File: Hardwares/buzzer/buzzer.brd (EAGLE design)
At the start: 95.5 x 82.6 mm, 5 parts, among them U1 ARDUINO-UNO-R3-SHIELD

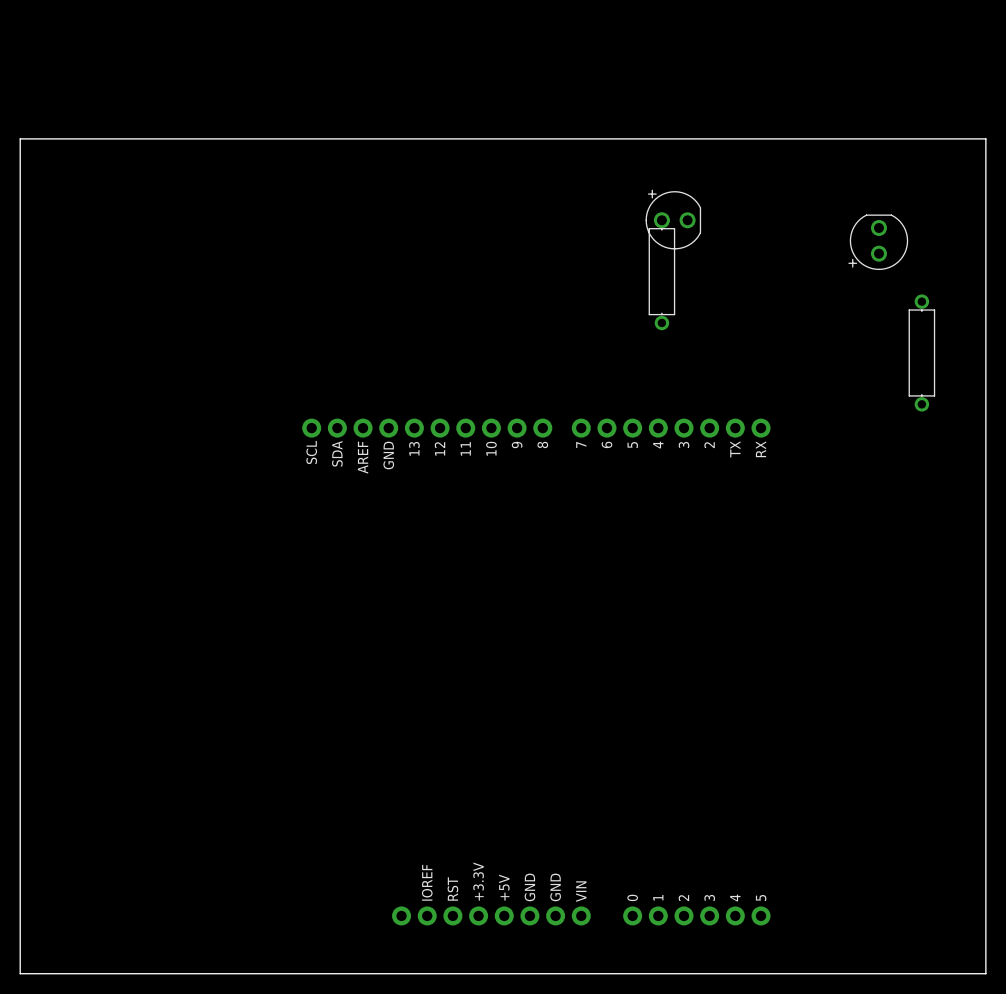
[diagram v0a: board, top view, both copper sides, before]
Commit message: brd csv html pdf png url ino
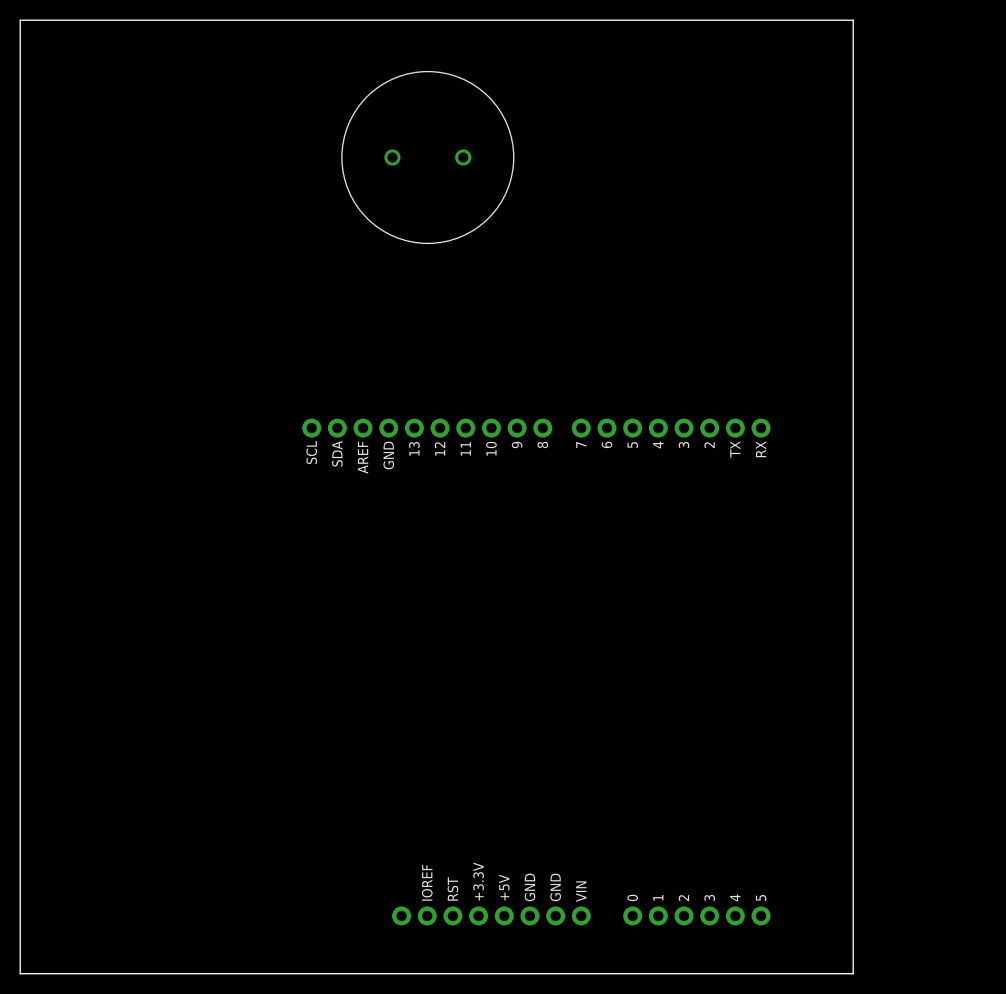
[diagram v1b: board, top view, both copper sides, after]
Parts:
- removed D1: GREEN, Tinkercad:LEDRD254W60D565H860B_G
- removed D2: RED, Tinkercad:LEDRD254W60D565H860B
- removed R1: 200, Tinkercad:RESAD1016W63L850D250B
- removed R2: 1k, Tinkercad:RESAD1016W63L850D250B
- added PIEZO1: PIEZO, Tinkercad:PIEZO
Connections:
- removed net D1_A: D1.1, R2.2
- removed net D2_A: D2.1, R1.1
- removed net U1_RX: R1.2, R2.1, U1.RX
- new net U1_D12: PIEZO1.1, U1.D12
- net U1_GND: now also PIEZO1.2; no longer D1.2, D2.2
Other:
- board size 95.5 x 82.6 mm -> 82.4 x 94.3 mm
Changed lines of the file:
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@@
 <board>
 <plain>
-<wire x1="0" y1="0" x2="95.52872003241336" y2="0" width="0" layer="20"/>
-<wire x1="95.52872003241336" y1="0" x2="95.52872003241336" y2="82.58300179113014" width="0" layer="20"/>
-<wire x1="95.52872003241336" y1="82.58300179113014" x2="0" y2="82.58300179113014" width="0" layer="20"/>
-<wire x1="0" y1="82.58300179113014" x2="0" y2="0" width="0" layer="20"/>
+<wire x1="0" y1="0" x2="82.40360000000003" y2="0" width="0" layer="20"/>
+<wire x1="82.40360000000003" y1="0" x2="82.40360000000003" y2="94.3253326403326" width="0" layer="20"/>
+<wire x1="82.40360000000003" y1="94.3253326403326" x2="0" y2="94.3253326403326" width="0" layer="20"/>
+<wire x1="0" y1="94.3253326403326" x2="0" y2="0" width="0" layer="20"/>
 </plain>
 <attributes/>
@@
 </autorouter>
 <elements>
-<element name="D2" library="Tinkercad" package="LEDRD254W60D565H860B" package3d_urn="urn:adsk.eagle:package:16378508/1" value="RED" x="64.7508" y="74.5334" rot="R360" smashed="yes">
-<attribute name="CATEGORY" value="Opto-Electronic" x="64.7508" y="74.5334" size="1.778" layer="27" display="off"/>
-<attribute name="COLOR" value="" x="64.7508" y="74.5334" size="1.778" layer="27" display="off"/>
-<attribute name="DESCRIPTION" value="" x="64.7508" y="74.5334" size="1.778" layer="27" display="off"/>
-<attribute name="MANUFACTURER" value="" x="64.7508" y="74.5334" size="1.778" layer="27" display="off"/>
-<attribute name="MPN" value="" x="64.7508" y="74.5334" size="1.778" layer="27" display="off"/>
-<attribute name="OPERATING_TEMP" value="" x="64.7508" y="74.5334" size="1.778" layer="27" display="off"/>
-<attribute name="PART_STATUS" value="" x="64.7508" y="74.5334" size="1.778" layer="27" display="off"/>
-<attribute name="ROHS_COMPLIANT" value="" x="64.7508" y="74.5334" size="1.778" layer="27" display="off"/>
-<attribute name="SERIES" value="" x="64.7508" y="74.5334" size="1.778" layer="27" display="off"/>
-<attribute name="SUB-CATEGORY" value="LED" x="64.7508" y="74.5334" size="1.778" layer="27" display="off"/>
-<attribute name="THERMALLOSS" value="" x="64.7508" y="74.5334" size="1.778" layer="27" display="off"/>
-<attribute name="TYPE" value="" x="64.7508" y="74.5334" size="1.778" layer="27" display="off"/>
-<attribute name="VALUE" value="LED_RED" x="64.7508" y="74.5334" size="1.778" layer="27" display="off"/>
-</element>
-<element name="R1" library="Tinkercad" package="RESAD1016W63L850D250B" package3d_urn="urn:adsk.eagle:package:31513020/1" value="200" x="63.4808" y="69.4534" rot="R270" smashed="yes"/>
+<element name="PIEZO1" library="Tinkercad" package="PIEZO" package3d_urn="urn:adsk.eagle:package:32623992/1" value="PIEZO" x="40.323" y="80.7453" rot="R180" smashed="yes"/>
 <element name="U1" library="Tinkercad" package="ARDUINO-UNO-R3-SHIELD" package3d_urn="urn:adsk.eagle:package:32092383/3" value="ARDUINO-UNO-R3-SHIELD" x="47.885" y="29.845" rot="R270" smashed="yes"/>
-<element name="D1" library="Tinkercad" package="LEDRD254W60D565H860B_G" package3d_urn="urn:adsk.eagle:package:31997108/2" value="GREEN" x="84.9537" y="72.5" rot="R90" smashed="yes">
-<attribute name="CATEGORY" value="Opto-Electronic" x="84.9537" y="72.5" size="1.778" layer="27" display="off"/>
-<attribute name="COLOR" value="" x="84.9537" y="72.5" size="1.778" layer="27" display="off"/>
-<attribute name="DESCRIPTION" value="" x="84.9537" y="72.5" size="1.778" layer="27" display="off"/>
-<attribute name="MANUFACTURER" value="" x="84.9537" y="72.5" size="1.778" layer="27" display="off"/>
-<attribute name="MPN" value="" x="84.9537" y="72.5" size="1.778" layer="27" display="off"/>
-<attribute name="OPERATING_TEMP" value="" x="84.9537" y="72.5" size="1.778" layer="27" display="off"/>
-<attribute name="PART_STATUS" value="" x="84.9537" y="72.5" size="1.778" layer="27" display="off"/>
-<attribute name="ROHS_COMPLIANT" value="" x="84.9537" y="72.5" size="1.778" layer="27" display="off"/>
-<attribute name="SERIES" value="" x="84.9537" y="72.5" size="1.778" layer="27" display="off"/>
-<attribute name="SUB-CATEGORY" value="LED" x="84.9537" y="72.5" size="1.778" layer="27" display="off"/>
-<attribute name="THERMALLOSS" value="" x="84.9537" y="72.5" size="1.778" layer="27" display="off"/>
-<attribute name="TYPE" value="" x="84.9537" y="72.5" size="1.778" layer="27" display="off"/>
-<attribute name="VALUE" value="LED_GREEN" x="84.9537" y="72.5" size="1.778" layer="27" display="off"/>
-</element>
-<element name="R2" library="Tinkercad" package="RESAD1016W63L850D250B" package3d_urn="urn:adsk.eagle:package:31513020/1" value="1k" x="89.1987" y="61.4056" rot="R90" smashed="yes"/>
 </elements>
 <signals>
 <signal name="U1_GND">
+<contactref element="PIEZO1" pad="2"/>
 <contactref element="U1" pad="GND@0"/>
 <contactref element="U1" pad="GND@1"/>
 <contactref element="U1" pad="GND@2"/>
-<contactref element="D2" pad="2"/>
-<contactref element="D1" pad="2"/>
 <wire x1="50.425" y1="5.715" x2="52.965" y2="5.715" width="0" layer="19" extent="1-1"/>
 <wire x1="50.425" y1="5.715" x2="36.455" y2="53.975" width="0" layer="19" extent="1-1"/>
-<wire x1="36.455" y1="53.975" x2="66.0208" y2="74.5334" width="0" layer="19" extent="1-1"/>
-<wire x1="66.0208" y1="74.5334" x2="84.9537" y2="73.77" width="0" layer="19" extent="1-1"/>
+<wire x1="36.823" y1="80.7453" x2="36.455" y2="53.975" width="0" layer="19" extent="1-1"/>
 </signal>
-<signal name="D2_A">
-<contactref element="R1" pad="1"/>
-<contactref element="D2" pad="1"/>
-<wire x1="63.4808" y1="74.5334" x2="63.4808" y2="74.5334" width="0" layer="19" extent="1-1"/>
-</signal>
-<signal name="U1_RX">
-<contactref element="R2" pad="1"/>
-<contactref element="R1" pad="2"/>
-<contactref element="U1" pad="RX"/>
-<wire x1="63.4808" y1="64.3734" x2="73.285" y2="53.975" width="0" layer="19" extent="1-1"/>
-<wire x1="89.1987" y1="56.3256" x2="73.285" y2="53.975" width="0" layer="19" extent="1-1"/>
-</signal>
-<signal name="D1_A">
-<contactref element="D1" pad="1"/>
-<contactref element="R2" pad="2"/>
-<wire x1="84.9537" y1="71.23" x2="89.1987" y2="66.4856" width="0" layer="19" extent="1-1"/>
+<signal name="U1_D12">
+<contactref element="PIEZO1" pad="1"/>
+<contactref element="U1" pad="D12"/>
+<wire x1="43.823" y1="80.7453" x2="41.535" y2="53.975" width="0" layer="19" extent="1-1"/>
 </signal>
 </signals>
